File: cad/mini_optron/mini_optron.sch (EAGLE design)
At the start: 10 parts

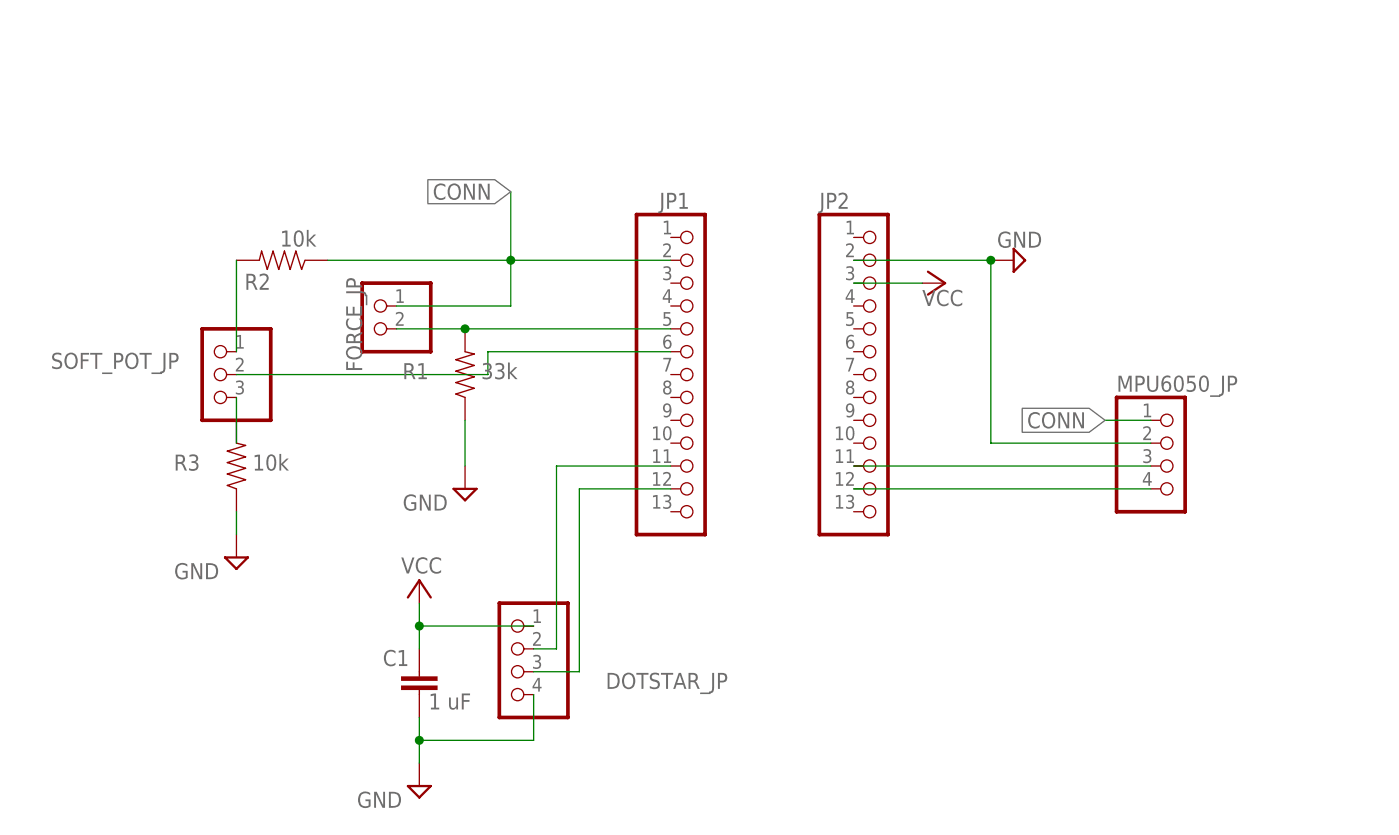
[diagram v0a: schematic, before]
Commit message: Add files via upload
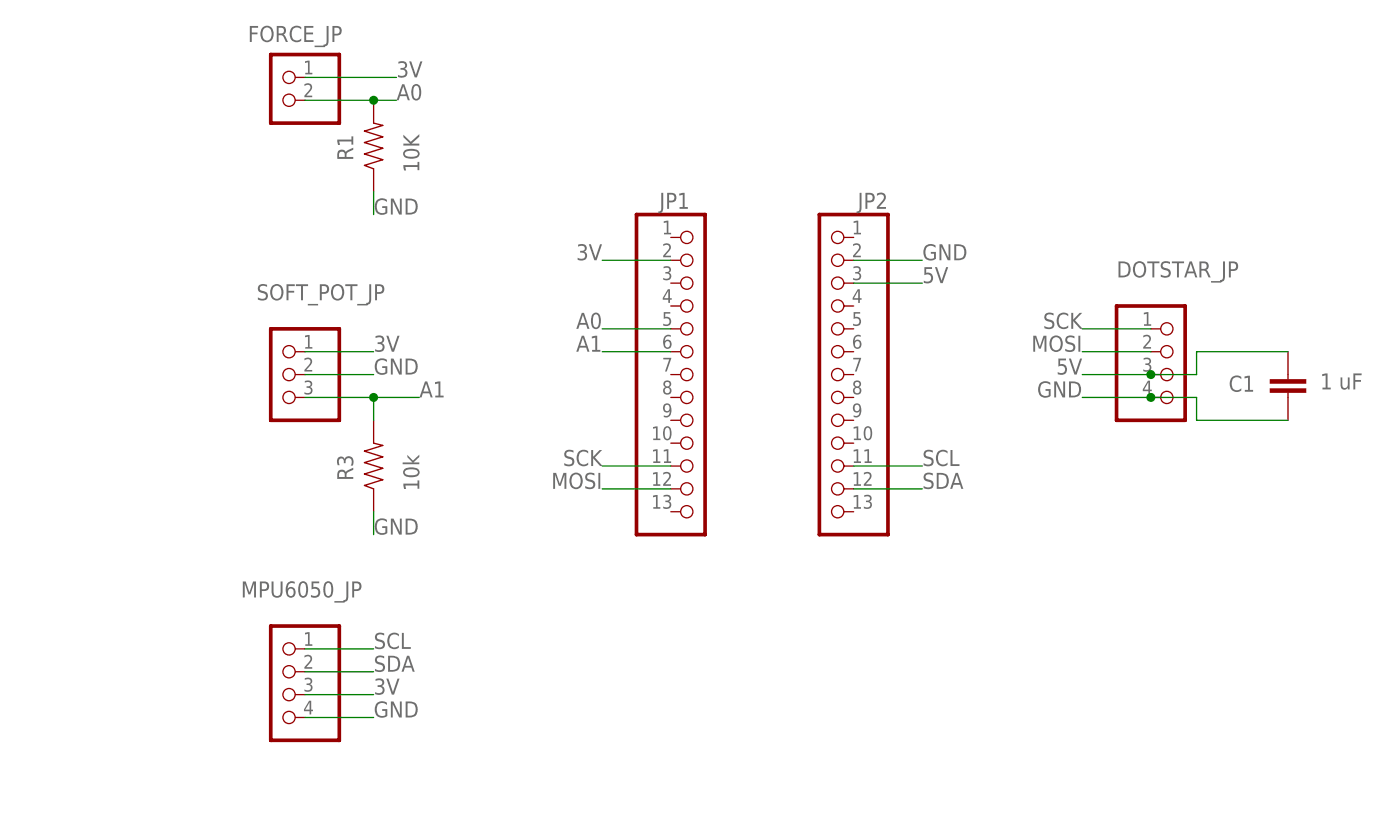
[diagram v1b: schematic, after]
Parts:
- removed R2: 10k, SparkFun-Resistors:RESISTORAXIAL-0.3
- R1: value 33k -> 10K
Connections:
- net N$1 renamed A0
- removed net CONN: FORCE_JP.1, JP1.2, MPU6050_JP.1, R2.1
- removed net N$10: JP2.12, MPU6050_JP.4
- removed net N$2: DOTSTAR_JP.2, JP1.11
- removed net N$3: R2.2, SOFT_POT_JP.1
- removed net N$4: JP1.6, SOFT_POT_JP.2
- removed net N$5: R3.2, SOFT_POT_JP.3
- removed net N$6: DOTSTAR_JP.3, JP1.12
- removed net N$9: JP2.11, MPU6050_JP.3
- removed net VCC: C1.1, DOTSTAR_JP.1, JP2.3
- new net 3V: FORCE_JP.1, JP1.2, MPU6050_JP.3, SOFT_POT_JP.1
- new net 5V: C1.1, DOTSTAR_JP.3, JP2.3
- new net A1: JP1.6, R3.2, SOFT_POT_JP.3
- new net MOSI: DOTSTAR_JP.2, JP1.12
- new net SCK: DOTSTAR_JP.1, JP1.11
- new net SCL: JP2.11, MPU6050_JP.1
- new net SDA: JP2.12, MPU6050_JP.2
- net GND: now also MPU6050_JP.4, SOFT_POT_JP.2; no longer MPU6050_JP.2
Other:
- moved on the sheet: C1, DOTSTAR_JP, FORCE_JP, MPU6050_JP, R1, R3, SOFT_POT_JP
